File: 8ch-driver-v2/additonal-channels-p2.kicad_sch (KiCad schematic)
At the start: 42 parts, among them Q6 2N7002E, Q7 2N7002E, Q8 2N7002E, U6 DRV104PWP, U7 DRV104PWP, U8 DRV104PWP

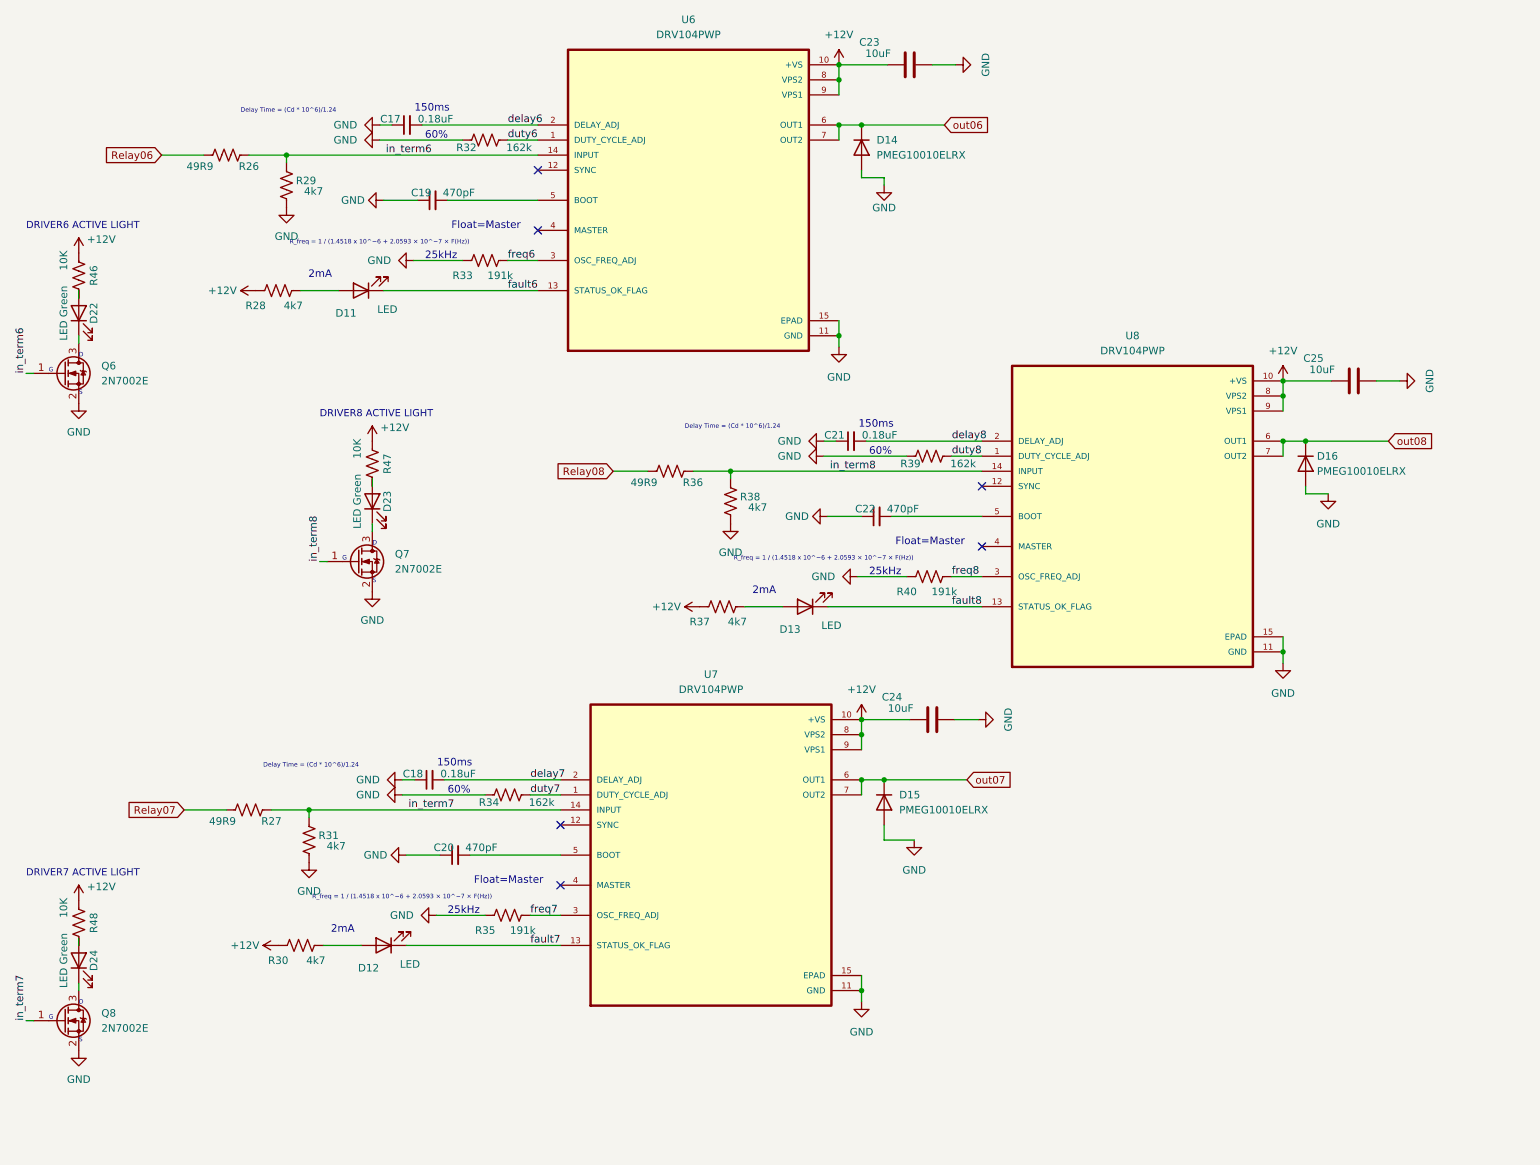
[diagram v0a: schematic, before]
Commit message: progress
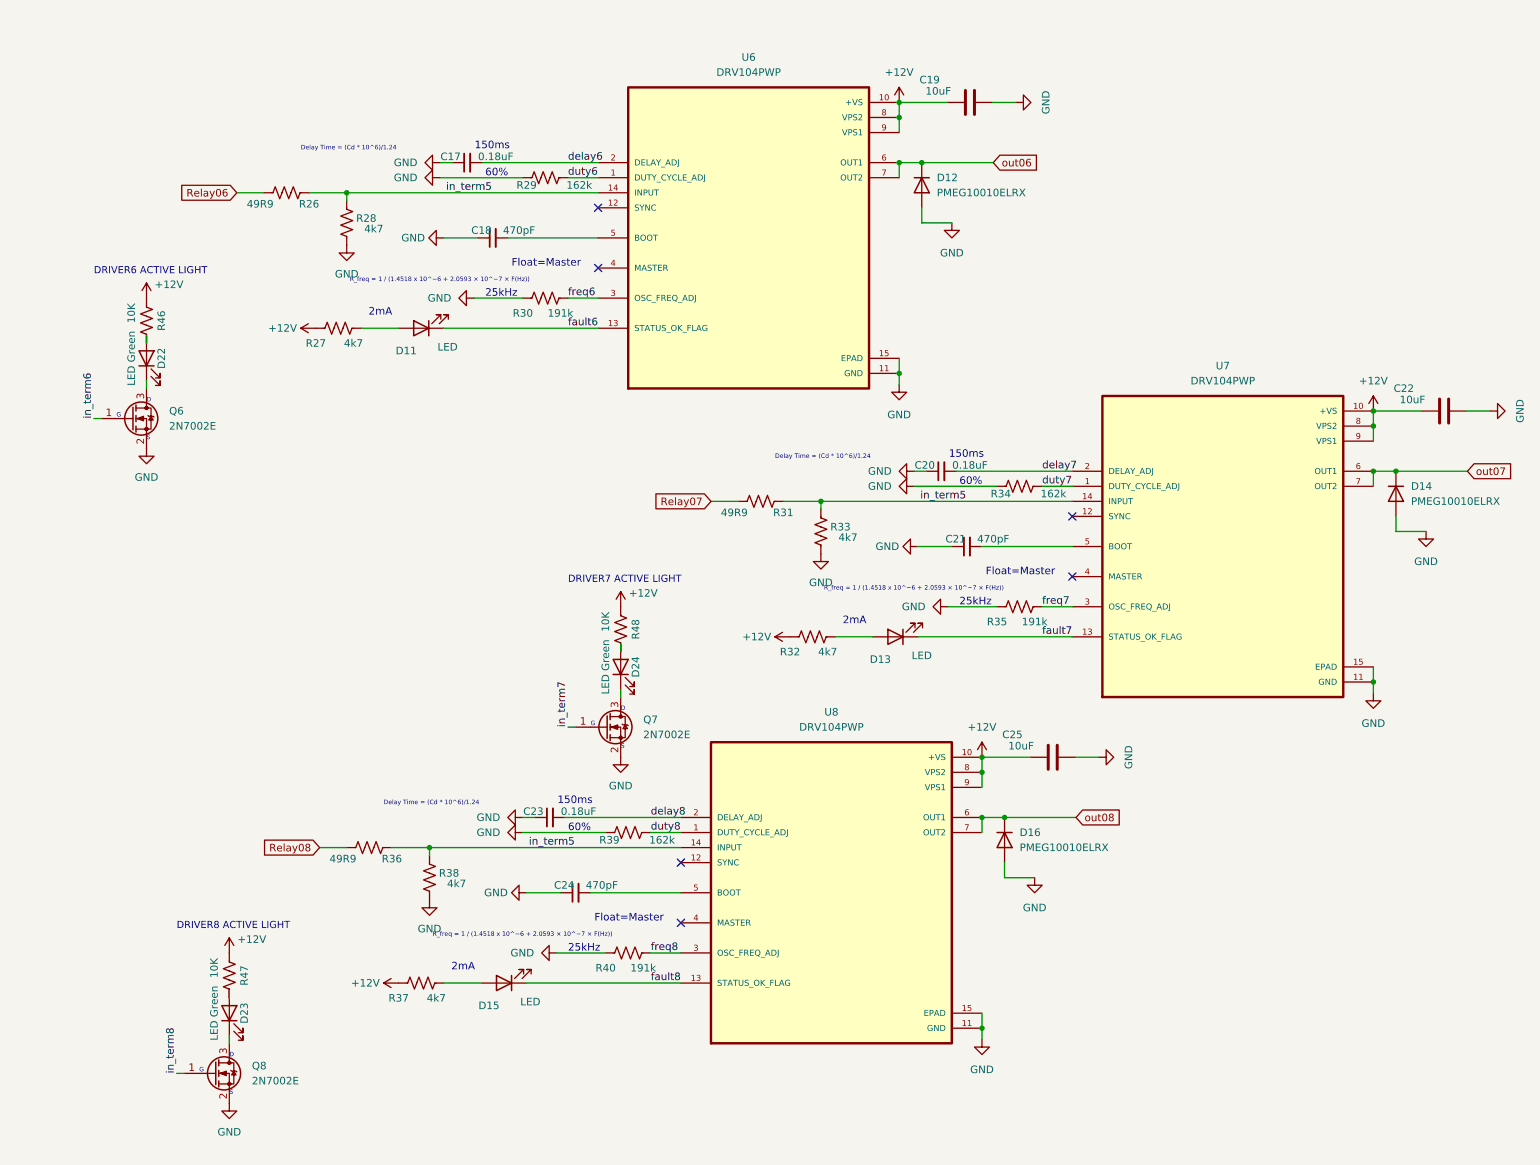
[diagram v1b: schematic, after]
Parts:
- removed C19, C22: 470pF, Capacitor_SMD:C_1206_3216Metric, symbol Device:C_Small
- removed C23, C24: 10uF, Capacitor_SMD:C_1210_3225Metric, symbol Device:C
- removed D12: LED, LED_SMD:LED_0805_2012Metric, symbol Device:LED
- removed D15: PMEG10010ELRX, Diode_SMD:Nexperia_CFP3_SOD-123W, symbol Device:D
- added C19, C22: 10uF, Capacitor_SMD:C_1210_3225Metric, symbol Device:C
- added C23: 0.18uF, Capacitor_SMD:C_1206_3216Metric, symbol Device:C_Small
- added C24: 470pF, Capacitor_SMD:C_1206_3216Metric, symbol Device:C_Small
- added D12: PMEG10010ELRX, Diode_SMD:Nexperia_CFP3_SOD-123W, symbol Device:D
- added D15: LED, LED_SMD:LED_0805_2012Metric, symbol Device:LED
- C18, C21: value 0.18uF -> 470pF; Mfg KYOCERA AVX -> Kemet; PartNum 08053C184KAT2A -> C0805C471K5RAC7800
- C20: value 470pF -> 0.18uF; Mfg Kemet -> KYOCERA AVX; PartNum C0805C471K5RAC7800 -> 08053C184KAT2A
- R27: value 49R9 -> 4k7; PartNum RC0805FR-0749R9L -> RC0805JR-074K7L
- R29: value 4k7 -> 162k; PartNum RC0805JR-074K7L -> RC0805FR-07162KL
- R30: value 4k7 -> 191k; PartNum RC0805JR-074K7L -> RC0805FR-07191KL
- R31: value 4k7 -> 49R9; PartNum RC0805JR-074K7L -> RC0805FR-0749R9L
- R32: value 162k -> 4k7; PartNum RC0805FR-07162KL -> RC0805JR-074K7L
- R33: value 191k -> 4k7; PartNum RC0805FR-07191KL -> RC0805JR-074K7L
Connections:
- net +12V: now also R27.1, R32.1, C19.1, C22.1; no longer R28.1, R30.1
- net GND: now also R28.1, R30.1, C19.2, C22.2, C23.1, C24.1, D12.2 (A); no longer R31.1, R32.1
- net Relay07: now also R31.1; no longer R27.1
- net delay7: now also C20.2; no longer C18.2
- net delay8: now also C23.2; no longer C21.2
- net duty6: now also R29.2; no longer R32.2
- net fault7: now also D13.1 (K)
- net fault8: now also D15.1 (K); no longer D13.1 (K)
- net freq6: now also R30.2; no longer R33.2
- net in_term6: no longer R26.2, R29.2, U6.14 (INPUT)
- net in_term7: now also Q7.1 (G); no longer Q8.1 (G), R27.2, R31.2, U7.14 (INPUT)
- net in_term8: now also Q8.1 (G); no longer Q7.1 (G), R36.2, R38.2, U8.14 (INPUT)
- net out06: now also D12.1 (K); no longer D14.1 (K)
- net out07: now also D14.1 (K)
- net at U7.5 (BOOT): now also C21.2; no longer C20.2
- net at U6.5 (BOOT): now also C18.2
- net at R37.2: now also D15.2 (A); no longer D13.2 (A)
- net at U8.5 (BOOT): now also C24.2
- net at Q8.3 (D): now also D23.1 (K); no longer D24.1 (K)
- net at Q7.3 (D): now also D24.1 (K); no longer D23.1 (K)
- net at D11.2 (A): now also R27.2; no longer R28.2
- new net: D13.2 (A), R32.2
- new net in_term5: R26.2, R28.2, R31.2, R33.2, R36.2, R38.2, U6.14 (INPUT), U7.14 (INPUT), U8.14 (INPUT)

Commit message: mucho mas progresso
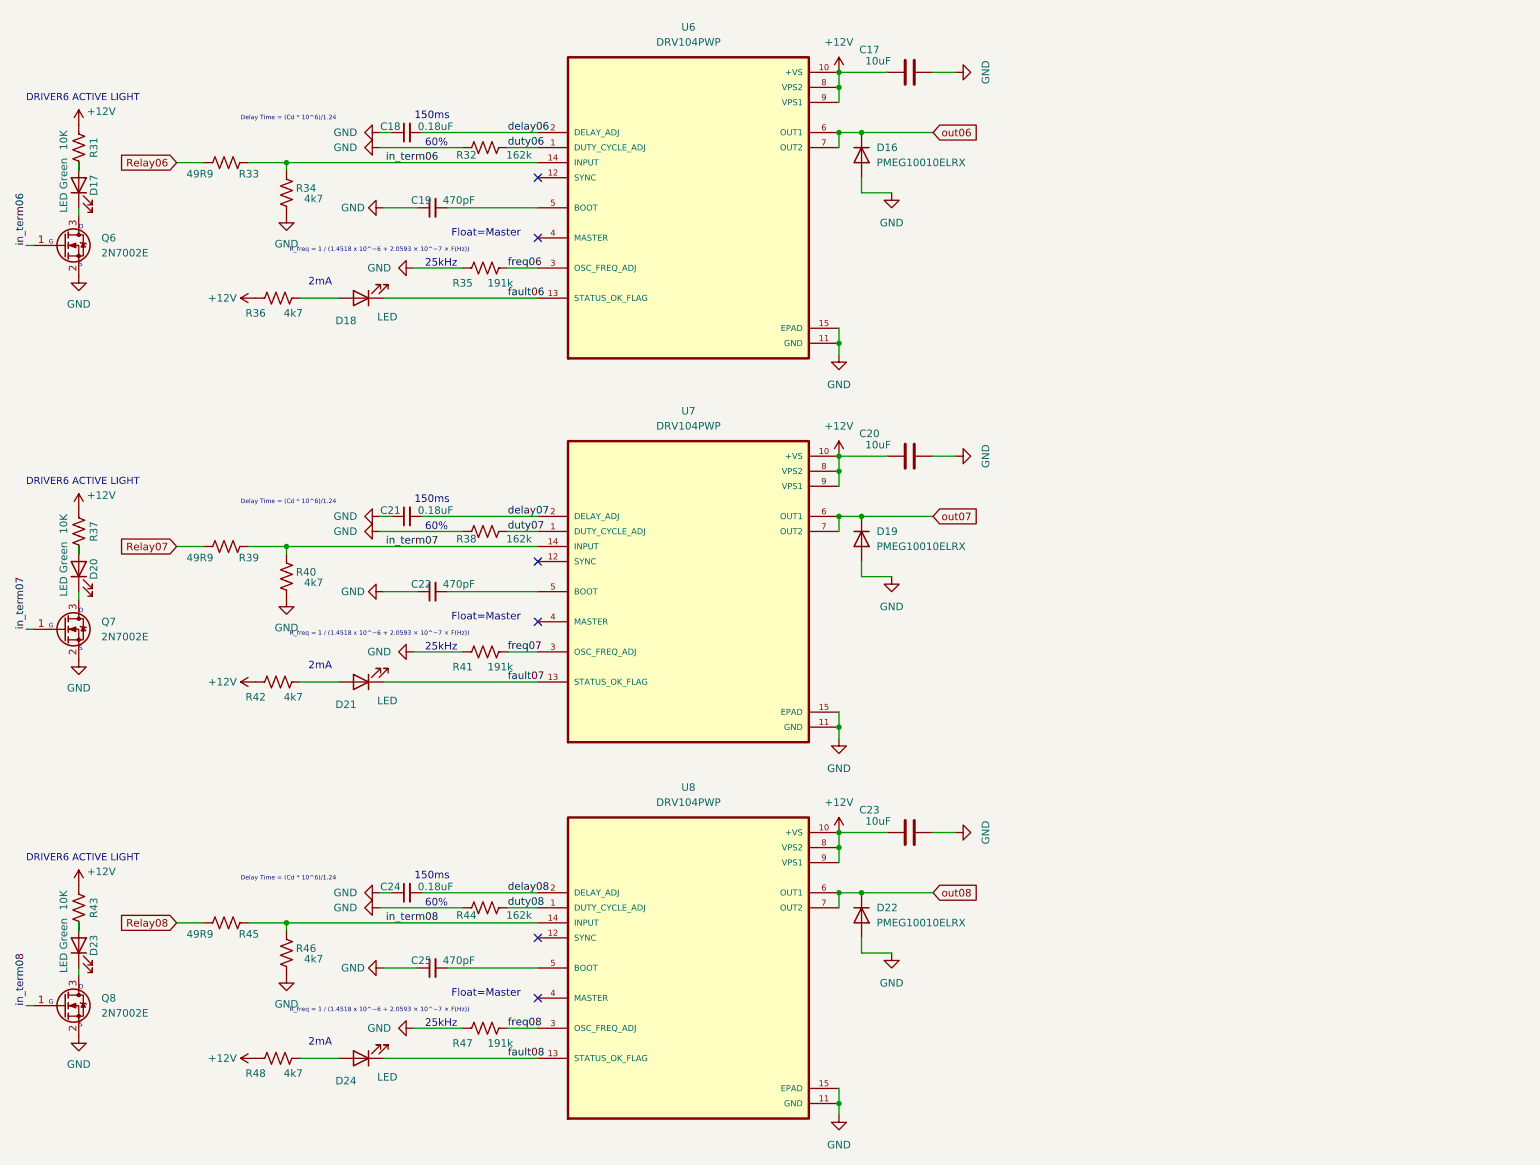
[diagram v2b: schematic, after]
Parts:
- removed C17, C20, C23: 0.18uF, Capacitor_SMD:C_1206_3216Metric, symbol Device:C_Small
- removed C19, C22, C25: 10uF, Capacitor_SMD:C_1210_3225Metric, symbol Device:C
- removed D11, D13, D15: LED, LED_SMD:LED_0805_2012Metric, symbol Device:LED
- removed D12, D14: PMEG10010ELRX, Diode_SMD:Nexperia_CFP3_SOD-123W, symbol Device:D
- removed D22: LED Green, LED_SMD:LED_0805_2012Metric, symbol Device:LED
- removed R26: 49R9, Resistor_SMD:R_1206_3216Metric, symbol Device:R_US
- removed R27, R28: 4k7, Resistor_SMD:R_1206_3216Metric, symbol Device:R_US
- removed R29: 162k, Resistor_SMD:R_1206_3216Metric, symbol Device:R_US
- removed R30: 191k, Resistor_SMD:R_1206_3216Metric, symbol Device:R_US
- added C17, C20, C23: 10uF, Capacitor_SMD:C_1210_3225Metric, symbol Device:C
- added C19, C22, C25: 470pF, Capacitor_SMD:C_1206_3216Metric, symbol Device:C_Small
- added D17, D20: LED Green, LED_SMD:LED_0805_2012Metric, symbol Device:LED
- added D18, D21: LED, LED_SMD:LED_0805_2012Metric, symbol Device:LED
- added D19, D22: PMEG10010ELRX, Diode_SMD:Nexperia_CFP3_SOD-123W, symbol Device:D
- added R41: 191k, Resistor_SMD:R_1206_3216Metric, symbol Device:R_US
- added R42: 4k7, Resistor_SMD:R_1206_3216Metric, symbol Device:R_US
- added R43: 10K, Resistor_SMD:R_1206_3216Metric, symbol Device:R_US
- added R44: 162k, Resistor_SMD:R_1206_3216Metric, symbol Device:R_US
- added R45: 49R9, Resistor_SMD:R_1206_3216Metric, symbol Device:R_US
- C18, C21, C24: value 470pF -> 0.18uF; Mfg Kemet -> KYOCERA AVX; PartNum C0805C471K5RAC7800 -> 08053C184KAT2A
- D24: value LED Green -> LED
- R31: value 49R9 -> 10K; PartNum RC0805FR-0749R9L -> RC0805FR-07162KL
- R32, R38: value 4k7 -> 162k; PartNum RC0805JR-074K7L -> RC0805FR-07162KL
- R33: value 4k7 -> 49R9; PartNum RC0805JR-074K7L -> RC0805FR-0749R9L
- R34: value 162k -> 4k7; PartNum RC0805FR-07162KL -> RC0805JR-074K7L
- R36: value 49R9 -> 4k7; PartNum RC0805FR-0749R9L -> RC0805JR-074K7L
- R37: value 4k7 -> 10K; PartNum RC0805JR-074K7L -> RC0805FR-07162KL
- R39: value 162k -> 49R9; PartNum RC0805FR-07162KL -> RC0805FR-0749R9L
- R40: value 191k -> 4k7; PartNum RC0805FR-07191KL -> RC0805JR-074K7L
- R46, R48: value 10K -> 4k7; PartNum RC0805FR-07162KL -> RC0805JR-074K7L
- R47: value 10K -> 191k; PartNum RC0805FR-07162KL -> RC0805FR-07191KL
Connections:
- net duty6 is gone; now on net duty06: U6.1 (DUTY_CYCLE_ADJ)
- net in_term8 is gone; now on net in_term08: Q8.1 (G)
- net +12V: now also R31.1, R36.1, C17.1, C20.1, C23.1, R42.1, R43.1; no longer R32.1, R46.1, R47.1
- net GND: now also R32.1, R46.1, R47.1, C17.2, C19.1, C20.2, C22.1, C23.2, C25.1, D19.2 (A), D22.2 (A), R41.1, R44.1; no longer R33.1, R39.1
- net Relay06: now also R33.1
- net Relay07: now also R39.1; no longer R31.1
- net Relay08: now also R45.1; no longer R36.1
- net out06: now also D16.1 (K)
- net out07: now also D19.1 (K)
- net out08: now also D22.1 (K); no longer D16.1 (K)
- net at R37.2: now also D20.2 (A)
- net at D23.2 (A): now also R43.2; no longer R47.2
- net duty06: now reaches R32.2
- net at U6.5 (BOOT): now also C19.2; no longer C18.2
- net in_term08: now reaches R46.2
- net in_term08: now also U8.14 (INPUT), R45.2
- net at U8.5 (BOOT): now also C25.2; no longer C24.2
- net at U7.5 (BOOT): now also C22.2; no longer C21.2
- net at Q6.3 (D): now also D17.1 (K)
- net at Q7.3 (D): now also D20.1 (K); no longer D24.1 (K)
- net delay6 renamed delay06
- net delay06: now also C18.2
- net delay7 renamed delay07
- net delay07: now also C21.2
- net delay8 renamed delay08
- net delay08: now also C24.2
- net duty7 renamed duty07
- net duty07: now also R38.2; no longer R34.2
- net duty8 renamed duty08
- net duty08: now also R44.2; no longer R39.2
- net fault6 renamed fault06
- net fault06: now also D18.1 (K)
- net fault7 renamed fault07
- net fault07: now also D21.1 (K)
- net fault8 renamed fault08
- net fault08: now also D24.1 (K)
- net freq6 renamed freq06
- net freq06: now also R35.2
- net freq7 renamed freq07
- net freq07: now also R41.2; no longer R35.2
- net freq8 renamed freq08
- net freq08: now also R47.2; no longer R40.2
- removed net in_term5: R31.2, R33.2, R36.2, R38.2, U6.14 (INPUT), U7.14 (INPUT), U8.14 (INPUT)
- net in_term6 renamed in_term06
- net in_term06: now also R33.2, R34.2, U6.14 (INPUT)
- net in_term7 renamed in_term07
- net in_term07: now also R39.2, R40.2, U7.14 (INPUT)
- new net: D21.2 (A), R42.2
- new net: D17.2 (A), R31.2
- new net: D18.2 (A), R36.2
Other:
- note removed: "DRIVER7 ACTIVE LIGHT"
- note removed: "DRIVER8 ACTIVE LIGHT"
